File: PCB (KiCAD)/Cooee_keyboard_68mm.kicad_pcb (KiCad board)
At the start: 2 copper layers, 66.8 x 41.8 mm, 110 parts, among them J9 Conn_01x05_Pin, U1 TCA8418RTWR

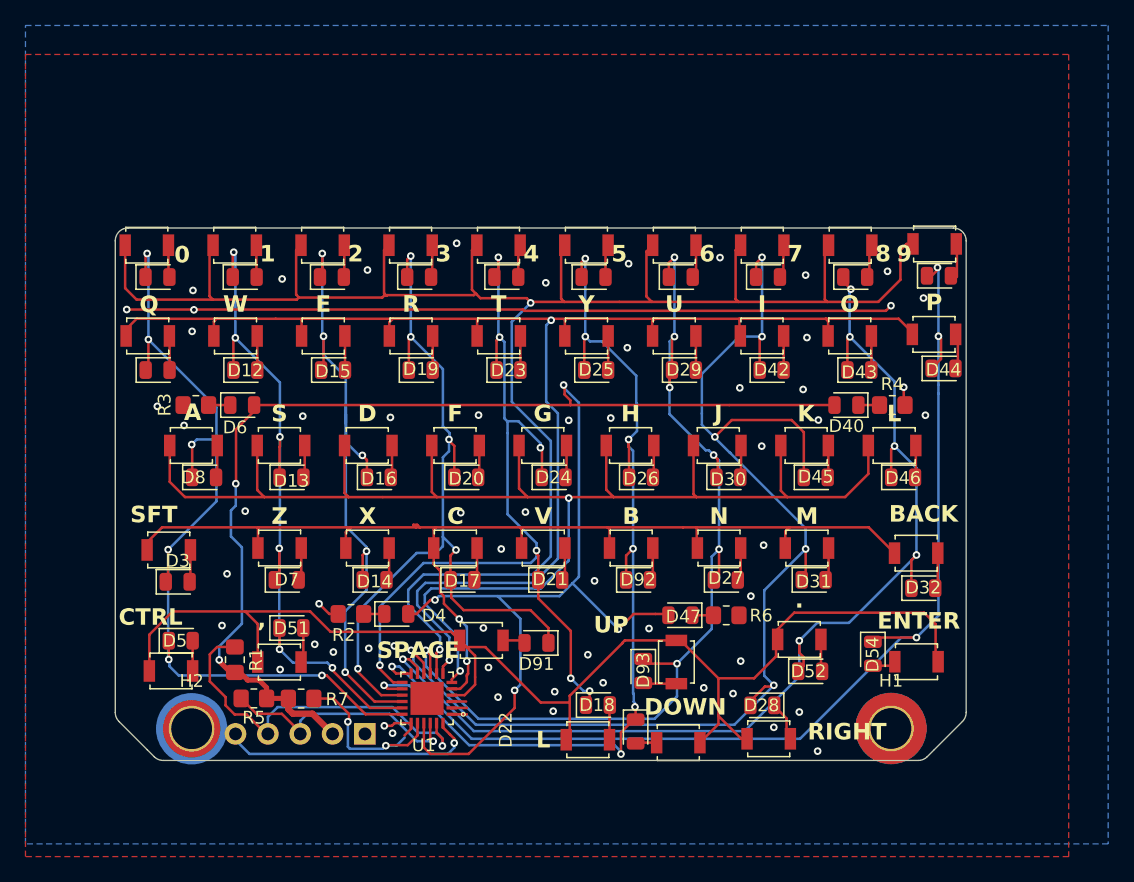
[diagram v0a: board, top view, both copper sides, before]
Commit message: pcb work
pcb work
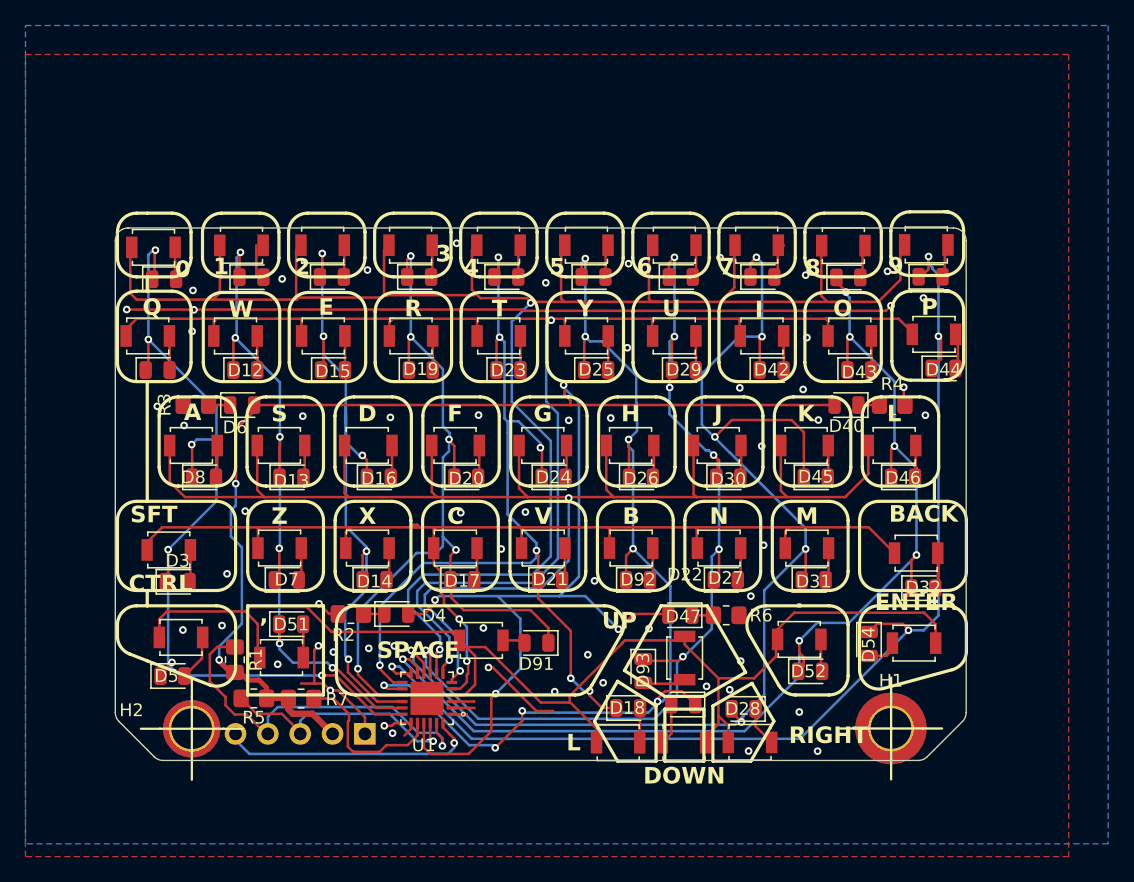
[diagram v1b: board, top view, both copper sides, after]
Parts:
- moved D22 4.30 mm to (161.4, 115.8), turned to 180 degrees
- moved D5 2.85 mm to (121.3, 113.6)
- moved SWe12 2.75 mm to (122.0, 110.5)
- moved D18 2.39 mm to (157.1, 116.1)
- moved SWe13 2.39 mm to (156.3, 118.8)
- moved D28 1.50 mm to (166.1, 116.2)
- moved SWe7 1.50 mm to (166.6, 118.8)
- moved SWe50 1.47 mm to (179.5, 111.0)
- moved D54 0.83 mm to (176.0, 111.1)
- moved SWe88 0.72 mm to (161.5, 112.2)
- moved D39 0.66 mm to (180.8, 82.2)
- moved SWe29 0.66 mm to (180.5, 79.7)
- moved D2 0.55 mm to (120.6, 82.4)
- moved ESC1 0.55 mm to (119.8, 79.9)
- moved D38 0.54 mm to (174.4, 82.3)
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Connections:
- ? pad 1: (no net) -> GND
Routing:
- net GND: track 67.9 -> 85.0 mm
- net COL6: track 74.7 -> 80.8 mm, vias 7 -> 8
- net ROW5: track 101.4 -> 97.3 mm
- net KEEB_RST: track 14.7 -> 13.0 mm, vias 2 -> 0
- net COL1: track 86.3 -> 88.0 mm
- net Net-(D22-A): track 1.68 -> 3.28 mm
- net COL3: track 98.9 -> 97.3 mm
- net ROW1: track 148.7 -> 147.2 mm
- net COL5: track 70.7 -> 72.2 mm
- net Net-(D5-A): track 2.38 -> 3.62 mm
- net COL10: track 69.4 -> 70.3 mm
- net Net-(D28-K): track 2.24 -> 3.15 mm
- net COL9: track 56.4 -> 55.6 mm
- net +3.3V: track 142.0 -> 142.8 mm
- net Net-(D93-A): track 2.63 -> 3.30 mm
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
